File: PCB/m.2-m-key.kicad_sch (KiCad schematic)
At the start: 16 parts, among them J1 Bus_M.2_Edge_M

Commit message: added the basic form factor
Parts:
- J1: footprint (none) -> FPGA:M.2 M-Key 2242
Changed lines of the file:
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@@
 			)
 		)
-		(property "Footprint" ""
+		(property "Footprint" "FPGA:M.2 M-Key 2242"
 			(at 162.56 85.09 0)
 			(effects

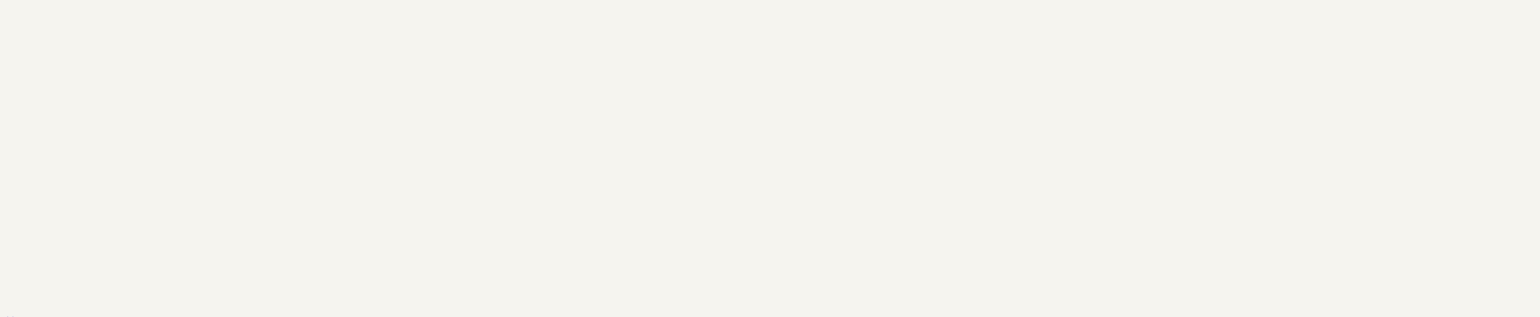
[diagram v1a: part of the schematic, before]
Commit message: finished add in all the footprints
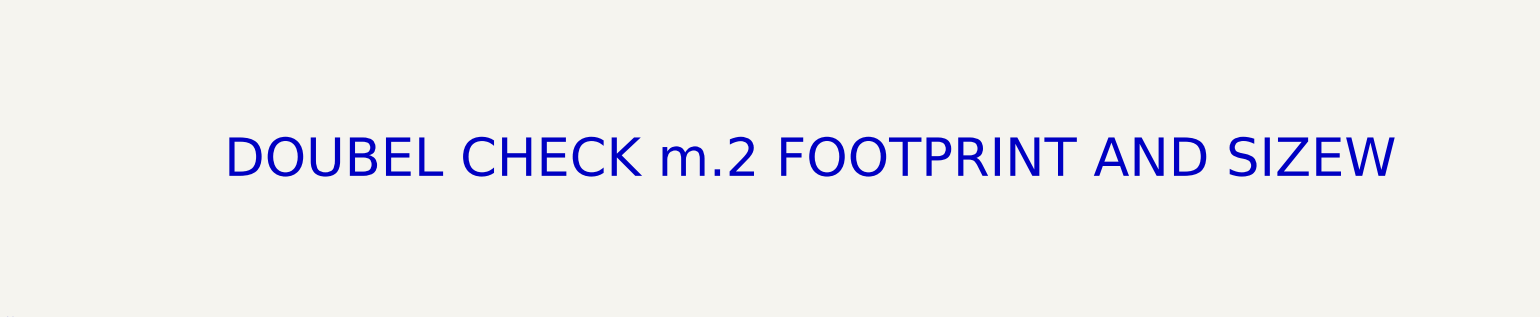
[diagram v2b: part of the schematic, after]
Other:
- note added: "DOUBEL CHECK m.2 FOOTPRINT AND SIZEW"
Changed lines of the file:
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@@
+		)
+	)
+	(text "DOUBEL CHECK m.2 FOOTPRINT AND SIZEW"
+		(exclude_from_sim no)
+		(at 363.22 107.696 0)
+		(effects
+			(font
+				(size 7.62 7.62)
+			)
 		)
 	)

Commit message: fixed my FPGA footprint for use with my symbol
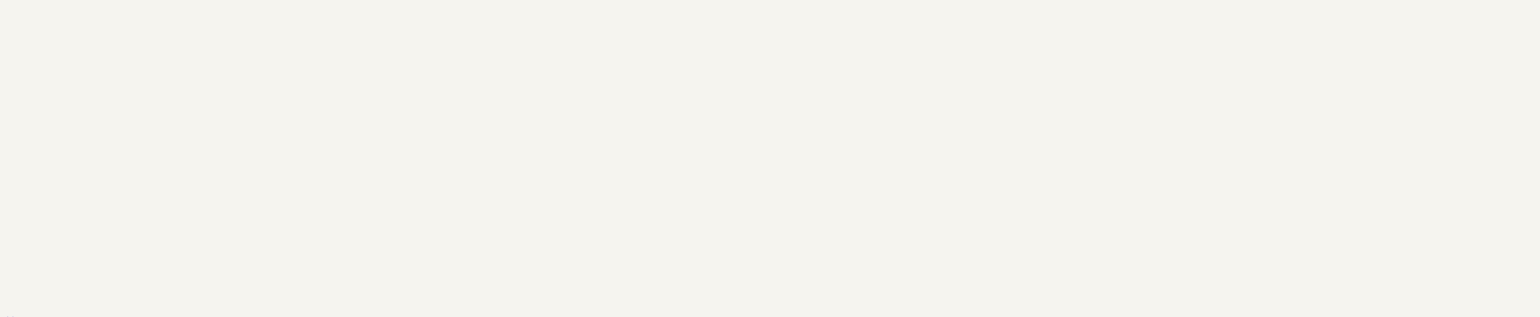
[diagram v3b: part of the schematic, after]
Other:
- note removed: "DOUBEL CHECK m.2 FOOTPRINT AND SIZEW"
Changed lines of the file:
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@@
-		)
-	)
-	(text "DOUBEL CHECK m.2 FOOTPRINT AND SIZEW"
-		(exclude_from_sim no)
-		(at 363.22 107.696 0)
-		(effects
-			(font
-				(size 7.62 7.62)
-			)
 		)
 	)
